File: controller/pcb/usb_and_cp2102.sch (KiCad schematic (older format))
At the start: 14 parts, among them P1 USB_C_Plug_USB2.0, Q5 BC817, Q6 BC817, U3 LM1117-3.3, U4 CP2102N-A01-GQFN24

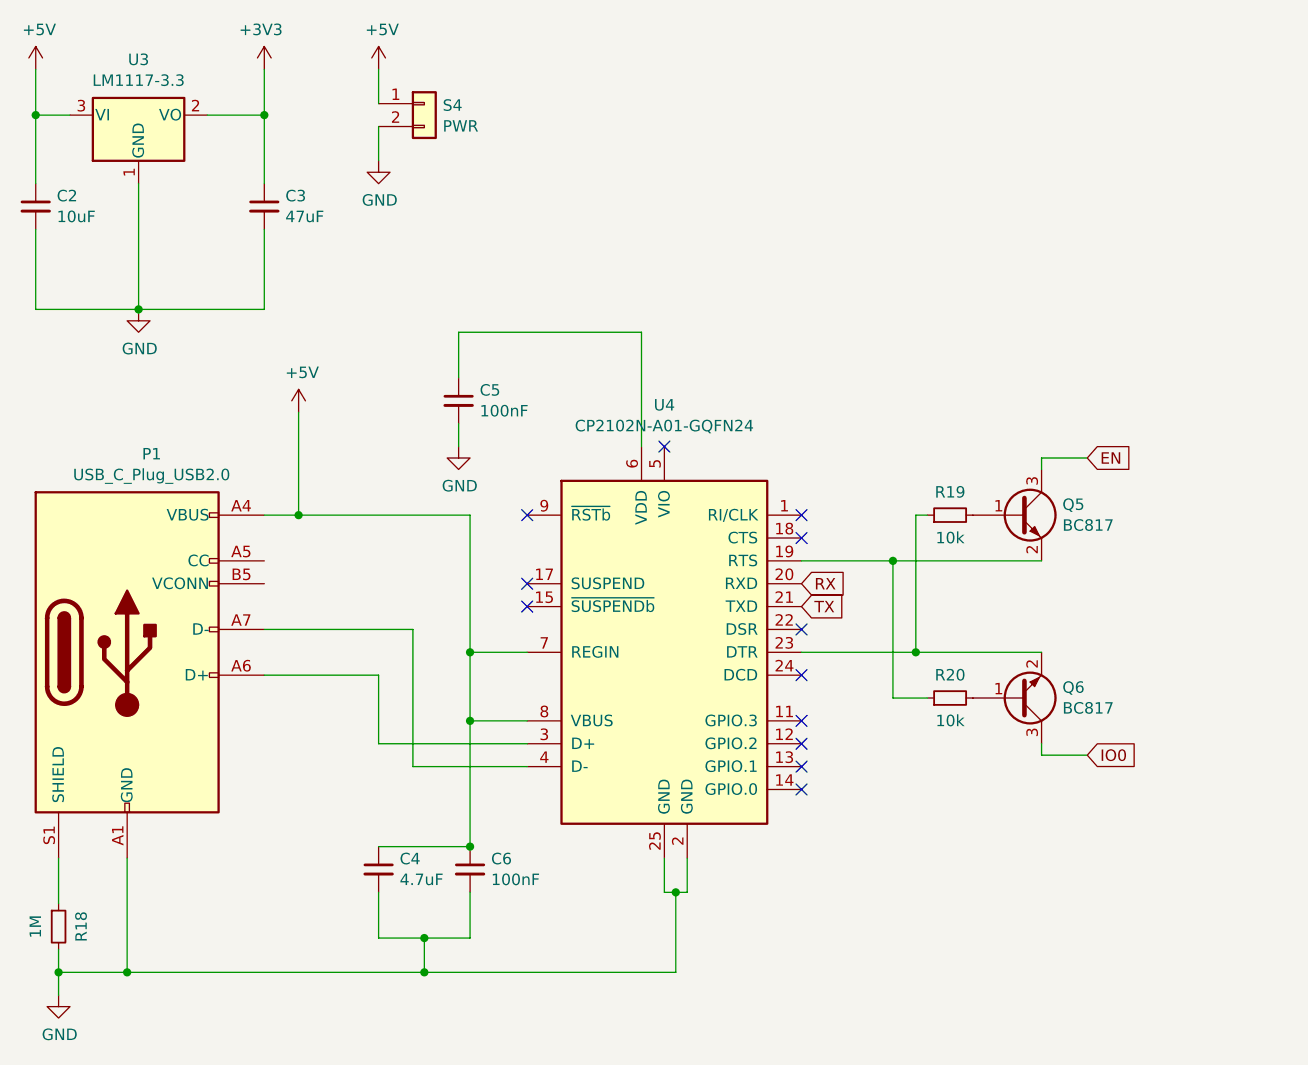
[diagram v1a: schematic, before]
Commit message: fix CP2102, minor bugs
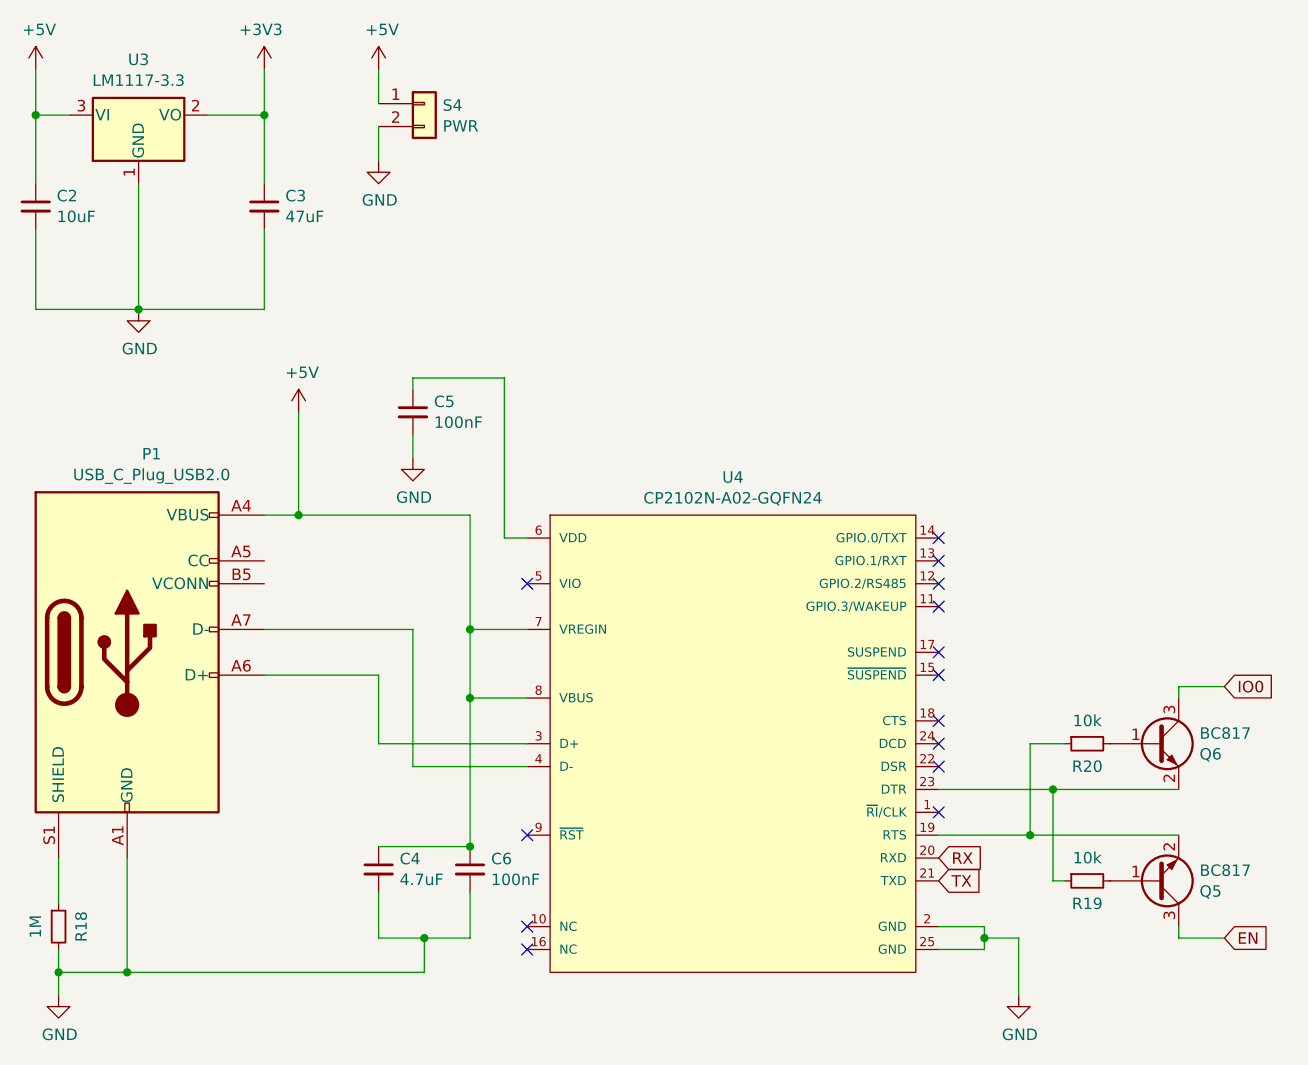
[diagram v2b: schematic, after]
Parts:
- removed U4: CP2102N-A01-GQFN24, Package_DFN_QFN:QFN-24-1EP_4x4mm_P0.5mm_EP2.6x2.6mm, symbol Interface_USB:CP2102N-A01-GQFN24
- added U4: CP2102N-A02-GQFN24, cp2102:Silicon_Labs-CP2102N-A02-GQFN24-IPC_A, symbol CP2102N-A02-GQFN24:CP2102N-A02-GQFN24
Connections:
- net +5V: now also U4.7 (VREGIN), U4.8 (VBUS)
- net GND: now also U4.2 (GND), U4.25 (GND)
- net RX: now also U4.20 (RXD)
- net TX: now also U4.21 (TXD)
- net at P1.A6 (D+): now also U4.3 (D+)
- net at P1.A7 (D-): now also U4.4 (D-)
- net at C5.1: now also U4.6 (VDD)
- net at Q5.2 (E), R20.1: now also U4.19 (RTS)
- net at Q6.2 (E), R19.1: now also U4.23 (DTR)
- no-connect marks 12 -> 14
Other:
- moved on the sheet: C5, Q5, Q6, R19, R20

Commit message: minor updates for cp2102
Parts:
- U4: symbol CP2102N-A02-GQFN24:CP2102N-A02-GQFN24 -> terrarium-rescue:CP2102N-A02-GQFN24-CP2102N-A02-GQFN24
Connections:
- net RX: now also U4.21 (TXD); no longer U4.20 (RXD)
- net TX: now also U4.20 (RXD); no longer U4.21 (TXD)
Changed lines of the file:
@@
 	1    0    0    1
 $EndComp
+Text GLabel 4900 4650 2    50   Input ~ 0
+RX
 Text GLabel 4900 4550 2    50   Input ~ 0
-RX
-Text GLabel 4900 4650 2    50   Input ~ 0
 TX
 $Comp
@@
 	2450 4050 3100 4050
 $Comp
-L CP2102N-A02-GQFN24:CP2102N-A02-GQFN24 U4
+L terrarium-rescue:CP2102N-A02-GQFN24-CP2102N-A02-GQFN24 U4
 U 1 1 61F6C1D8
 P 3000 3150
+AR Path="/61F6C1D8" Ref="U4"  Part="1"
+AR Path="/623D759E/61F6C1D8" Ref="U4"  Part="1"
 F 0 "U4" H 4000 3415 50  0000 C CNN
 F 1 "CP2102N-A02-GQFN24" H 4000 3324 50  0000 C CNN
